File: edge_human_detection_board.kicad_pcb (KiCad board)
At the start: 4 copper layers, 4 parts, among them IC1 TXB0108PWR

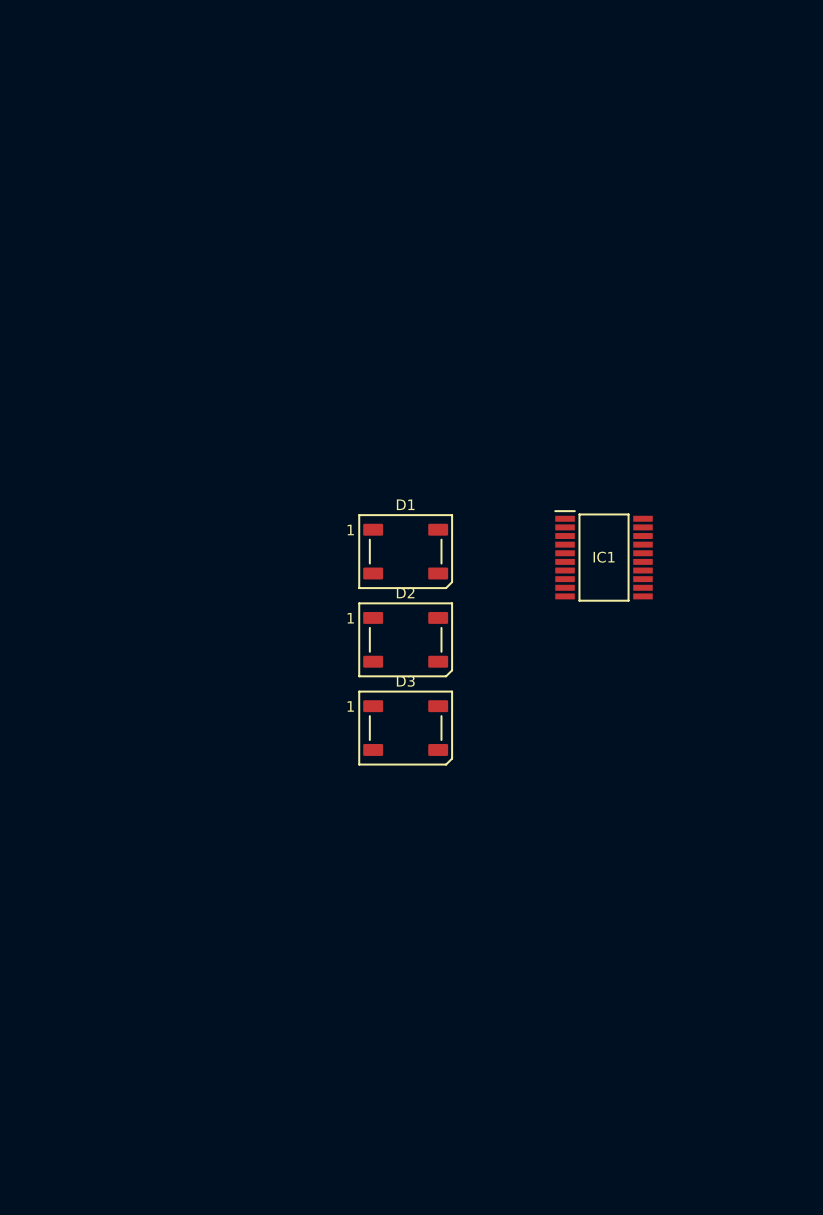
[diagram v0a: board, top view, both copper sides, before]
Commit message: working on board
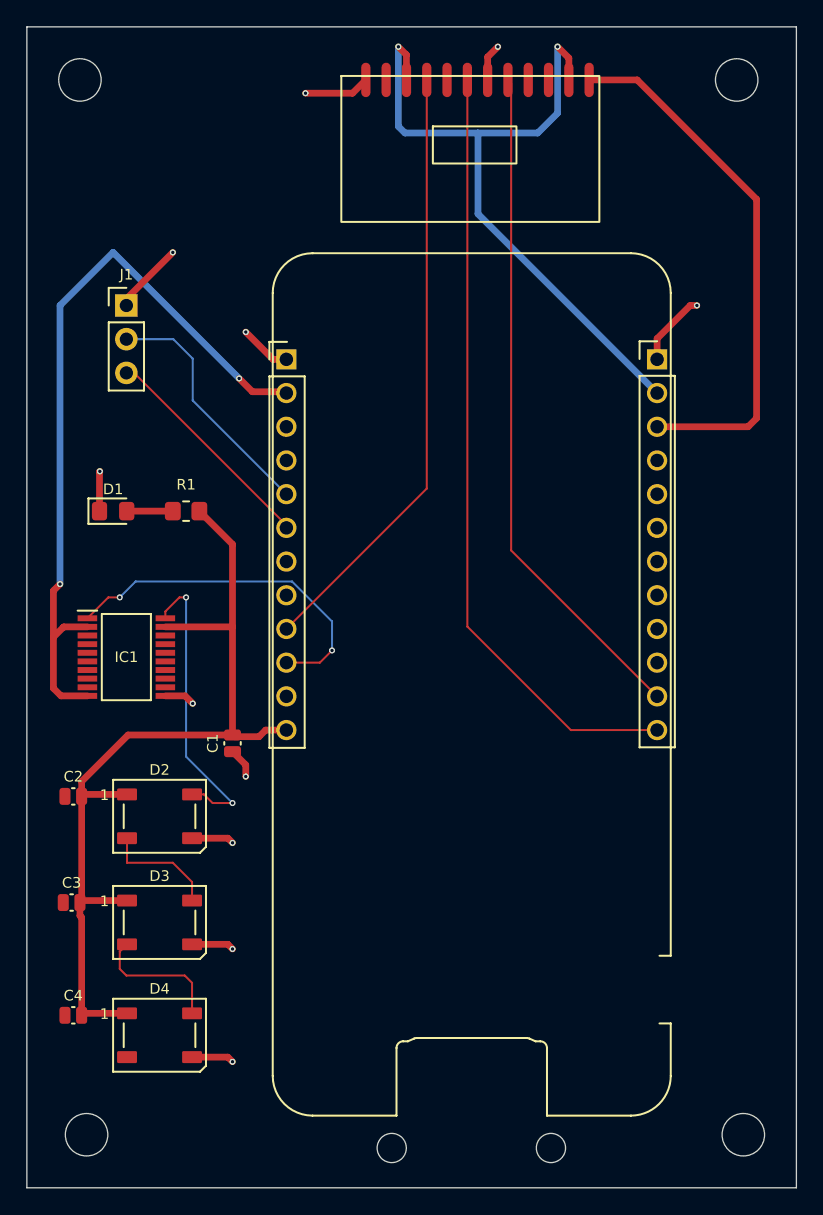
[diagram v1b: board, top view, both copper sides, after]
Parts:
- added C1: 0.1uF, Capacitor_SMD:C_0504_1310Metric_Pad0.83x1.28mm_HandSolder, F.Cu at (130.0, 87.0)
- added C2: 0.1uF, Capacitor_SMD:C_0504_1310Metric_Pad0.83x1.28mm_HandSolder, F.Cu at (118.0, 91.0)
- added C3: 0.1uF, Capacitor_SMD:C_0504_1310Metric_Pad0.83x1.28mm_HandSolder, F.Cu at (117.9, 99.0)
- added C4: 0.1uF, Capacitor_SMD:C_0504_1310Metric_Pad0.83x1.28mm_HandSolder, F.Cu at (118.0, 107.5)
- added D4: WS2812B, LED_SMD:LED_WS2812B_PLCC4_5.0x5.0mm_P3.2mm, F.Cu at (124.5, 109.0)
- added J1: Conn_01x03_Socket, Connector_PinHeader_2.54mm:PinHeader_1x03_P2.54mm_Vertical, F.Cu at (122.0, 54.0)
- added R1: 1.5k, Resistor_SMD:R_0805_2012Metric_Pad1.20x1.40mm_HandSolder, F.Cu at (126.5, 69.5)
- added REF**: MountingHole_2.2mm_M2, MountingHole:MountingHole_2.2mm_M2, F.Cu at (142.0, 117.5)
- added REF**: MountingHole_3.2mm_M3, MountingHole:MountingHole_3.2mm_M3, F.Cu at (168.5, 116.5)
- added REF**: MountingHole_3.2mm_M3, MountingHole:MountingHole_3.2mm_M3, F.Cu at (119.0, 116.5)
- added REF**: MountingHole_2.2mm_M2, MountingHole:MountingHole_2.2mm_M2, F.Cu at (154.0, 117.5)
- added REF**: MountingHole_3.2mm_M3, MountingHole:MountingHole_3.2mm_M3, F.Cu at (118.5, 37.0)
- added REF**: MountingHole_3.2mm_M3, MountingHole:MountingHole_3.2mm_M3, F.Cu at (168.0, 37.0)
- added U1: ~, 00_parts_lib:coral_micro_board_mating, F.Cu at (149.9, 79.2)
- added U2: ~, 00_parts_lib:SATEL-VL53L8A, F.Cu at (148.0, 41.2)
- D1: value WS2812B -> LED; footprint LED_SMD:LED_WS2812B_PLCC4_5.0x5.0mm_P3.2mm -> LED_SMD:LED_0805_2012Metric_Pad1.15x1.40mm_HandSolder
- moved IC1 36.8 mm to (122.0, 80.5)
- moved D3 23.6 mm to (124.5, 100.5)
- moved D2 22.8 mm to (124.5, 92.5)
- moved D1 22.3 mm to (121.0, 69.5)
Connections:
- D1 pad 1: /Coral Micro Breakouts/+5VDC -> GND
- D1 pad 2: Net-(D1-DOUT) -> Net-(D1-A)
- D2 pad 4: Net-(D1-DOUT) -> Net-(D2-DIN)
- D3 pad 2: unconnected-(D3-DOUT-Pad2) -> Net-(D3-DOUT)
- IC1 pad 20: Net-(D1-DIN) -> Net-(D2-DIN)
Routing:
- net /Coral Micro Breakouts/+5VDC: track 0.00 -> 68.4 mm
- net /Coral Micro Breakouts/SDA: track 0.00 -> 58.7 mm
- net /Coral Micro Breakouts/+1.8VDC_RGB: track 0.00 -> 57.8 mm, vias 0 -> 2
- net /Coral Micro Breakouts/+1.8VDC_TOF: track 0.00 -> 54.6 mm, vias 0 -> 2
- net /Coral Micro Breakouts/SCL: track 0.00 -> 51.1 mm
- net /Coral Micro Breakouts/PWM_1: track 0.00 -> 45.8 mm
- net /Coral Micro Breakouts/+3.3VDC: track 0.00 -> 40.6 mm
- net GND: track 0.00 -> 39.9 mm, vias 0 -> 11
- net /Coral Micro Breakouts/PWM_0: track 0.00 -> 26.8 mm, vias 0 -> 2
- net Net-(D2-DIN): track 0.00 -> 22.8 mm, vias 0 -> 2
- net /Coral Micro Breakouts/DEBUG_TX: track 0.00 -> 18.7 mm
- net /Coral Micro Breakouts/DEBUG_RX: track 0.00 -> 17.7 mm
- net Net-(D3-DOUT): track 0.00 -> 10.3 mm
- net Net-(D2-DOUT): track 0.00 -> 8.75 mm
- net Net-(D1-A): track 0.00 -> 3.47 mm
- added copper zone on In1.Cu, net GND
- added copper zone on In2.Cu, net GND
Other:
- board outline added: 58 x 87.5 mm
- board text added: "EDGE DETECTION BOARD REV 1.0.0 BY JC"
